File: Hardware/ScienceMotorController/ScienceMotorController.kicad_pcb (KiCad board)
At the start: 2 copper layers, 124.5 x 119.6 mm, 122 parts, among them U1 OKI, U2 TM4C129E_Launchpad, U3 VNH5019A_E, U4 VNH5019A_E, U5 VNH5019A_E, U6 VNH5019A_E, U7 VNH5019A_E, U8 VNH5019A_E

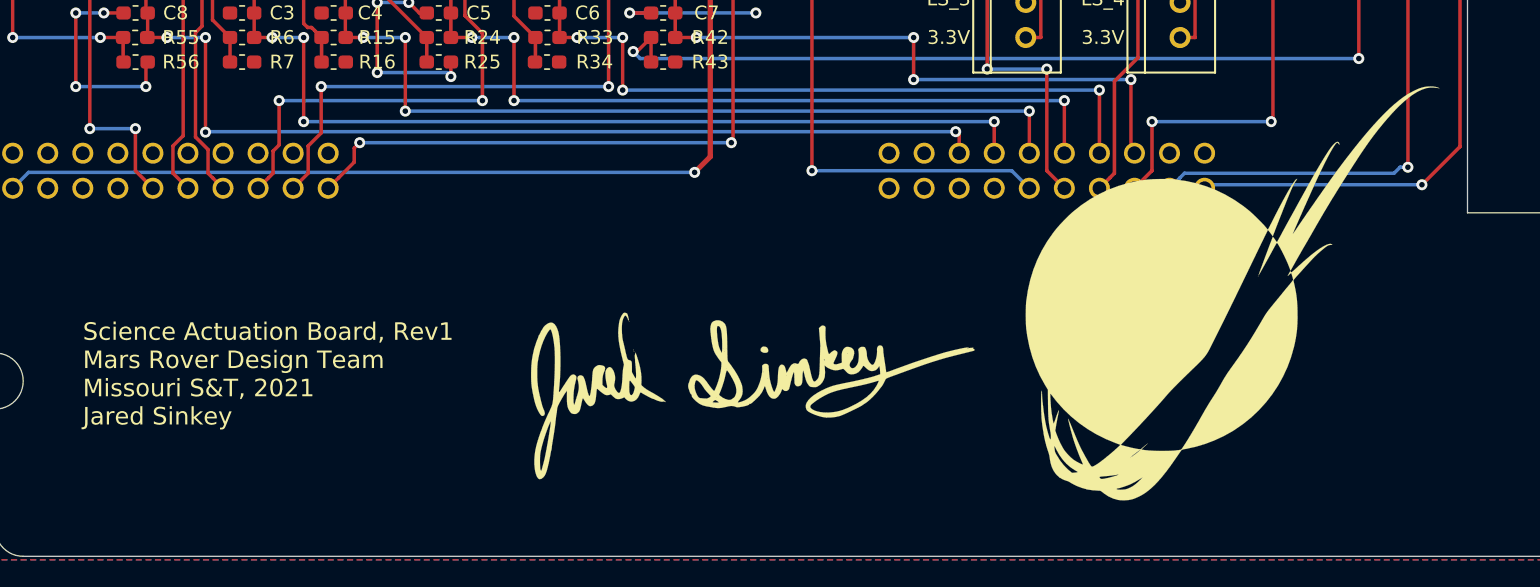
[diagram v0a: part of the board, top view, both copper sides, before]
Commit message: Added Gerbs
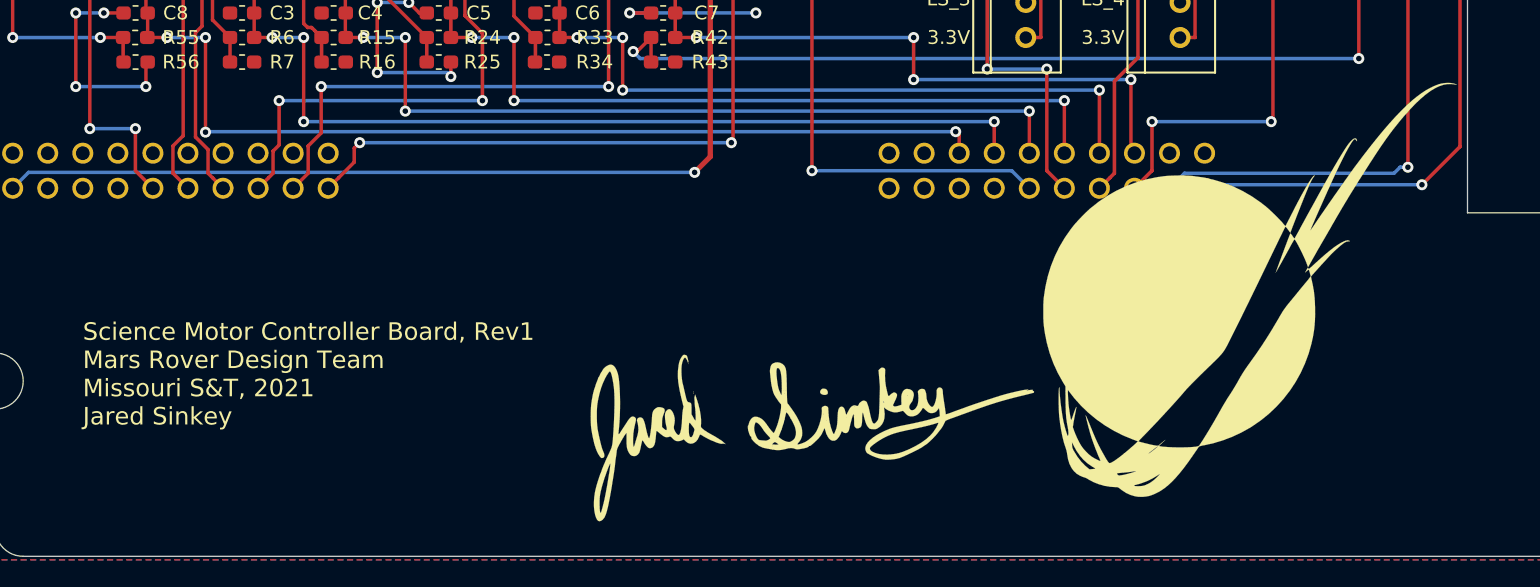
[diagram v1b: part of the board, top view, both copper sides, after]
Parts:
- moved G*** 5.29 mm to (94.0, 149.9)
- moved G*** 1.30 mm to (125.5, 139.7)
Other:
- board text added: "Science Motor Controller Board, Rev1 Mars Rover Design Team Missouri S&T, 2021 Jared Sinkey"
- board text removed: "Science Actuation Board, Rev1 Mars Rover Design Team Missouri S&T, 2021 Jared Sinkey"
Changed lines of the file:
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@@
       (outputformat 1)
       (mirror false)
-      (drillshape 1)
+      (drillshape 0)
       (scaleselection 1)
-      (outputdirectory ""))
+      (outputdirectory "Gerbs/"))
   )
   (net 0 "")
@@
   )
   (module MRDT_Silkscreens:z_sig_Jared_Sinkey_15.5mmx34.4mm (layer F.Cu)
-    (at 89.662 146.812 90)
+    (at 93.98 149.86 90)
     (fp_text reference G*** (at 0 0 90) (layer F.SilkS) hide
       (effects (font (size 1.524 1.524) (thickness 0.3)))
@@
   )
   (module MRDT_Silkscreens:0_MRDT_Logo_30mm (layer F.Cu)
-    (at 124.206 139.954)
+    (at 125.476 139.7)
     (tags "Logo, MRDT")
     (fp_text reference G*** (at -4.6228 17.8054) (layer Dwgs.User) hide
@@
     (effects (font (size 1 1) (thickness 0.15)))
   )
-  (gr_text "Science Actuation Board, Rev1\nMars Rover Design Team\nMissouri S&T, 2021\nJared Sinkey" (at 40.894 145.796) (layer F.SilkS)
+  (gr_text "Science Motor Controller Board, Rev1\nMars Rover Design Team\nMissouri S&T, 2021\nJared Sinkey" (at 40.894 145.796) (layer F.SilkS)
     (effects (font (size 1.27 1.27) (thickness 0.15)) (justify left))
   )
